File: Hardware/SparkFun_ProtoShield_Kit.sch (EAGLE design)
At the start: 25 parts

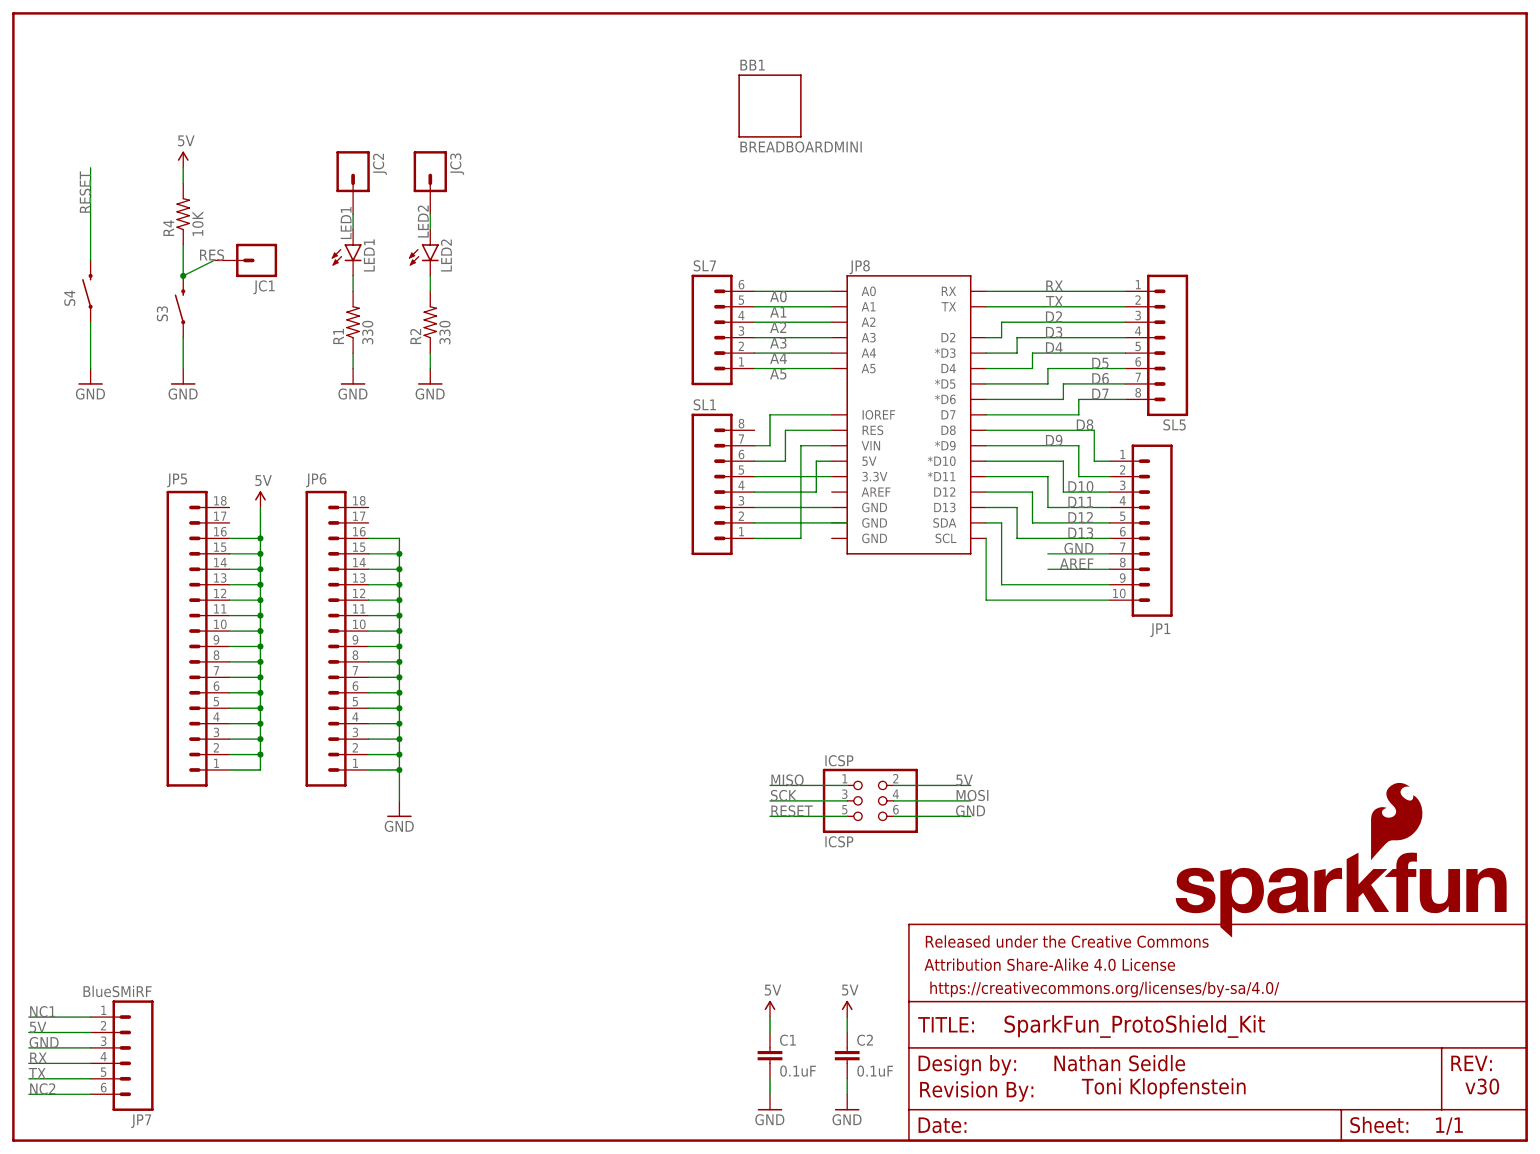
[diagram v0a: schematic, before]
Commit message: Ready for engineering review
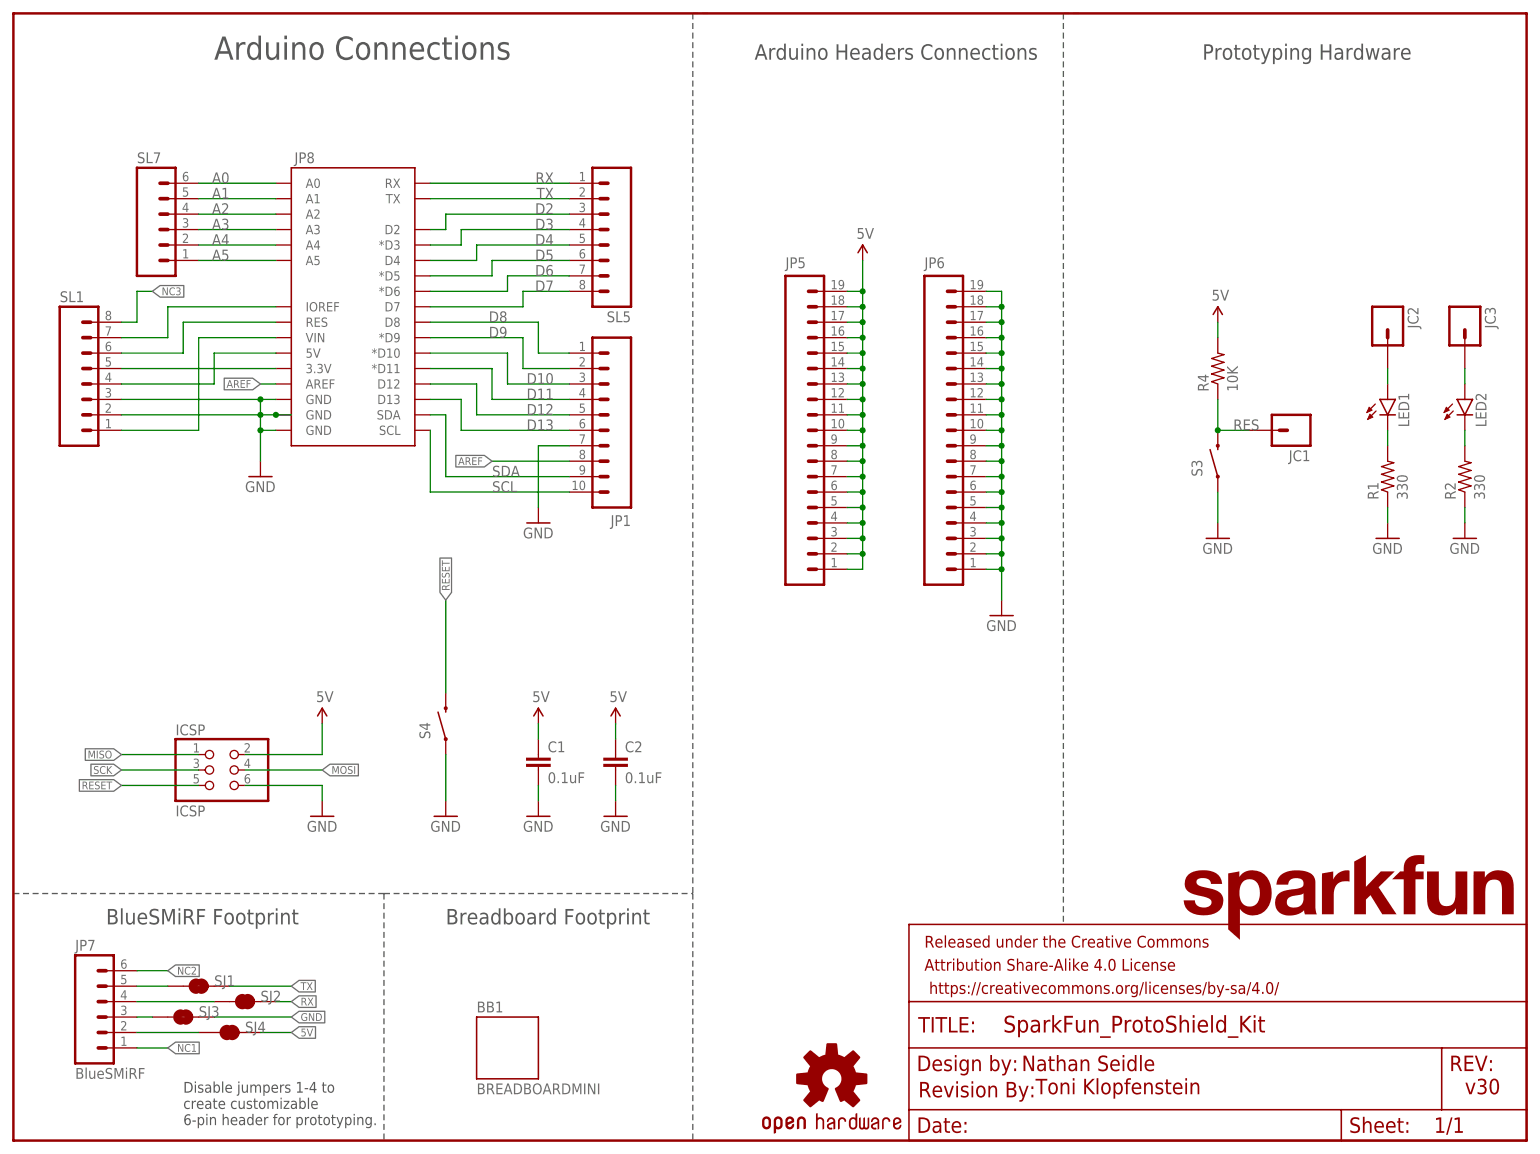
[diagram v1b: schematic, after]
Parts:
- added LOGO1: OSHW-LOGOS, SparkFun-Aesthetics:OSHW-LOGOS
- added SJ1, SJ2, SJ3, SJ4: JUMPER-PAD-2-NC_BY_TRACE, SparkFun-Passives:JUMPER-PAD-2-NC_BY_TRACE
- JP5, JP6: device TempLibrary:M18" -> SparkFun-Connectors:M191X19
- U$1: value SFE_LOGO_NAME_FLAME.1_INCH -> SFE_LOGO_NAME.1_INCH; device SparkFun-Aesthetics:SFE_LOGO_NAME_FLAME.1_INCH -> SparkFun-Aesthetics:SFE_LOGO_NAME.1_INCH
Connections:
- net N$186 renamed SDA
- net N$187 renamed SCL
- removed net N$183: JP8.GND@2, SL1.3
- removed net N$184: SL1.2
- new net N$219: JP7.3, SJ3.1
- new net N$220: JP7.2, SJ4.1
- new net NC3: SL1.8
- net 5V: now also JP5.17, JP5.18, JP5.19, JP8.5V, SJ4.2, SL1.4; no longer JP7.2
- net AREF: now also JP8.AREF
- net GND: now also JP6.17, JP6.18, JP6.19, JP8.GND@0, JP8.GND@1, JP8.GND@2, SJ3.2, SL1.2, SL1.3; no longer JP7.3
- net N$2: now also JP7.5, SJ1.1; no longer JP8.RES, SL1.6
- net N$9: now also JP7.4, SJ2.1; no longer JP8.5V, SL1.4
- net RESET: now also JP8.RES, SL1.6
- net RX: now also SJ2.2; no longer JP7.4
- net TX: now also SJ1.2; no longer JP7.5
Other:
- note added: "Arduino Connections"
- note added: "Arduino Headers Connections"
- note added: "BlueSMiRF Footprint"
- note added: "Breadboard Footprint"
- note added: "Disable jumpers 1-4 to create customizable 6-pin header for prototyping."
- note added: "Prototyping Hardware"
- moved on the sheet: BB1, C1, C2, ICSP, JC1, JC2, JC3, JP1, JP7, JP8, LED1, LED2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
